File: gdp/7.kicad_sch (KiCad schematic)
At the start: 8 parts, among them IC1 74LS74, IC15A 74LS367, IC2 74LS42, IC21 74LS374, IC28 74LS374, IC35 74LS374, IC48 74LS374, IC9 74LS374

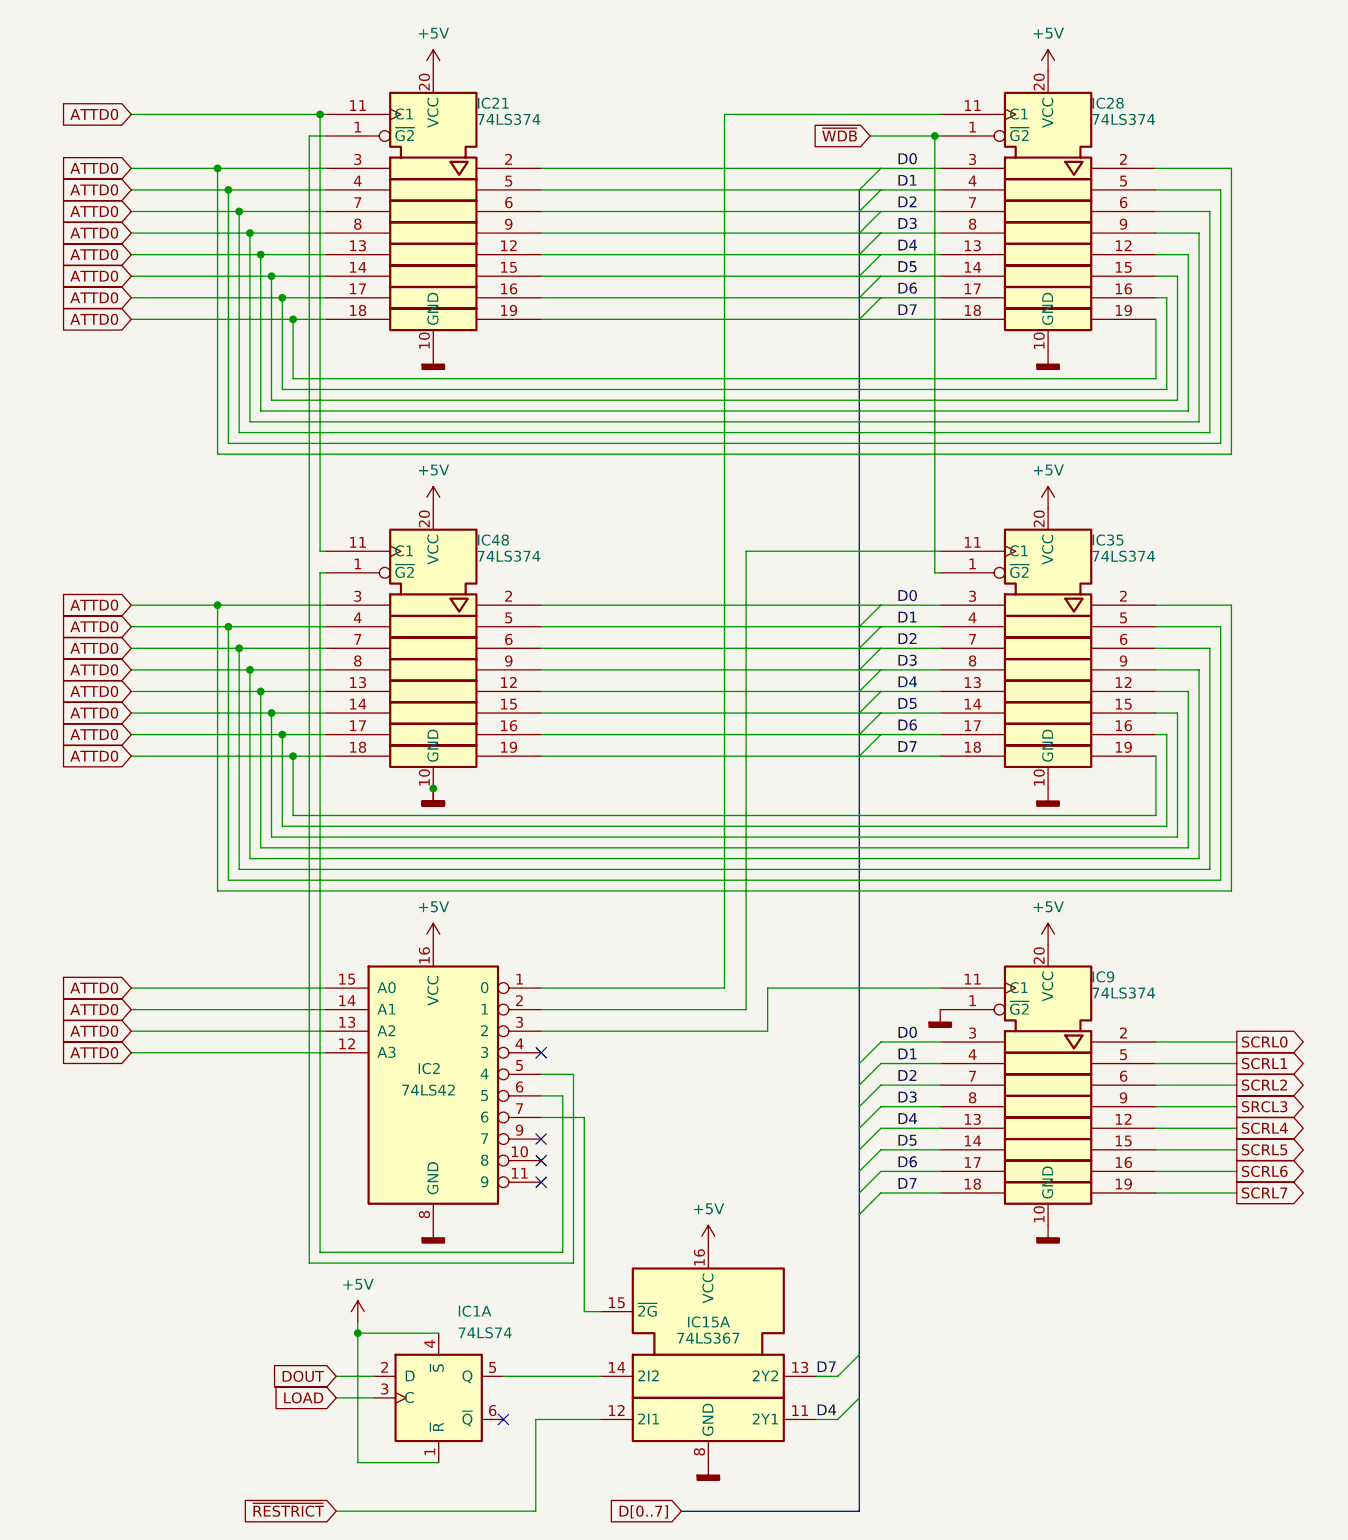
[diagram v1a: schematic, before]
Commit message: Fixes Sheet 7
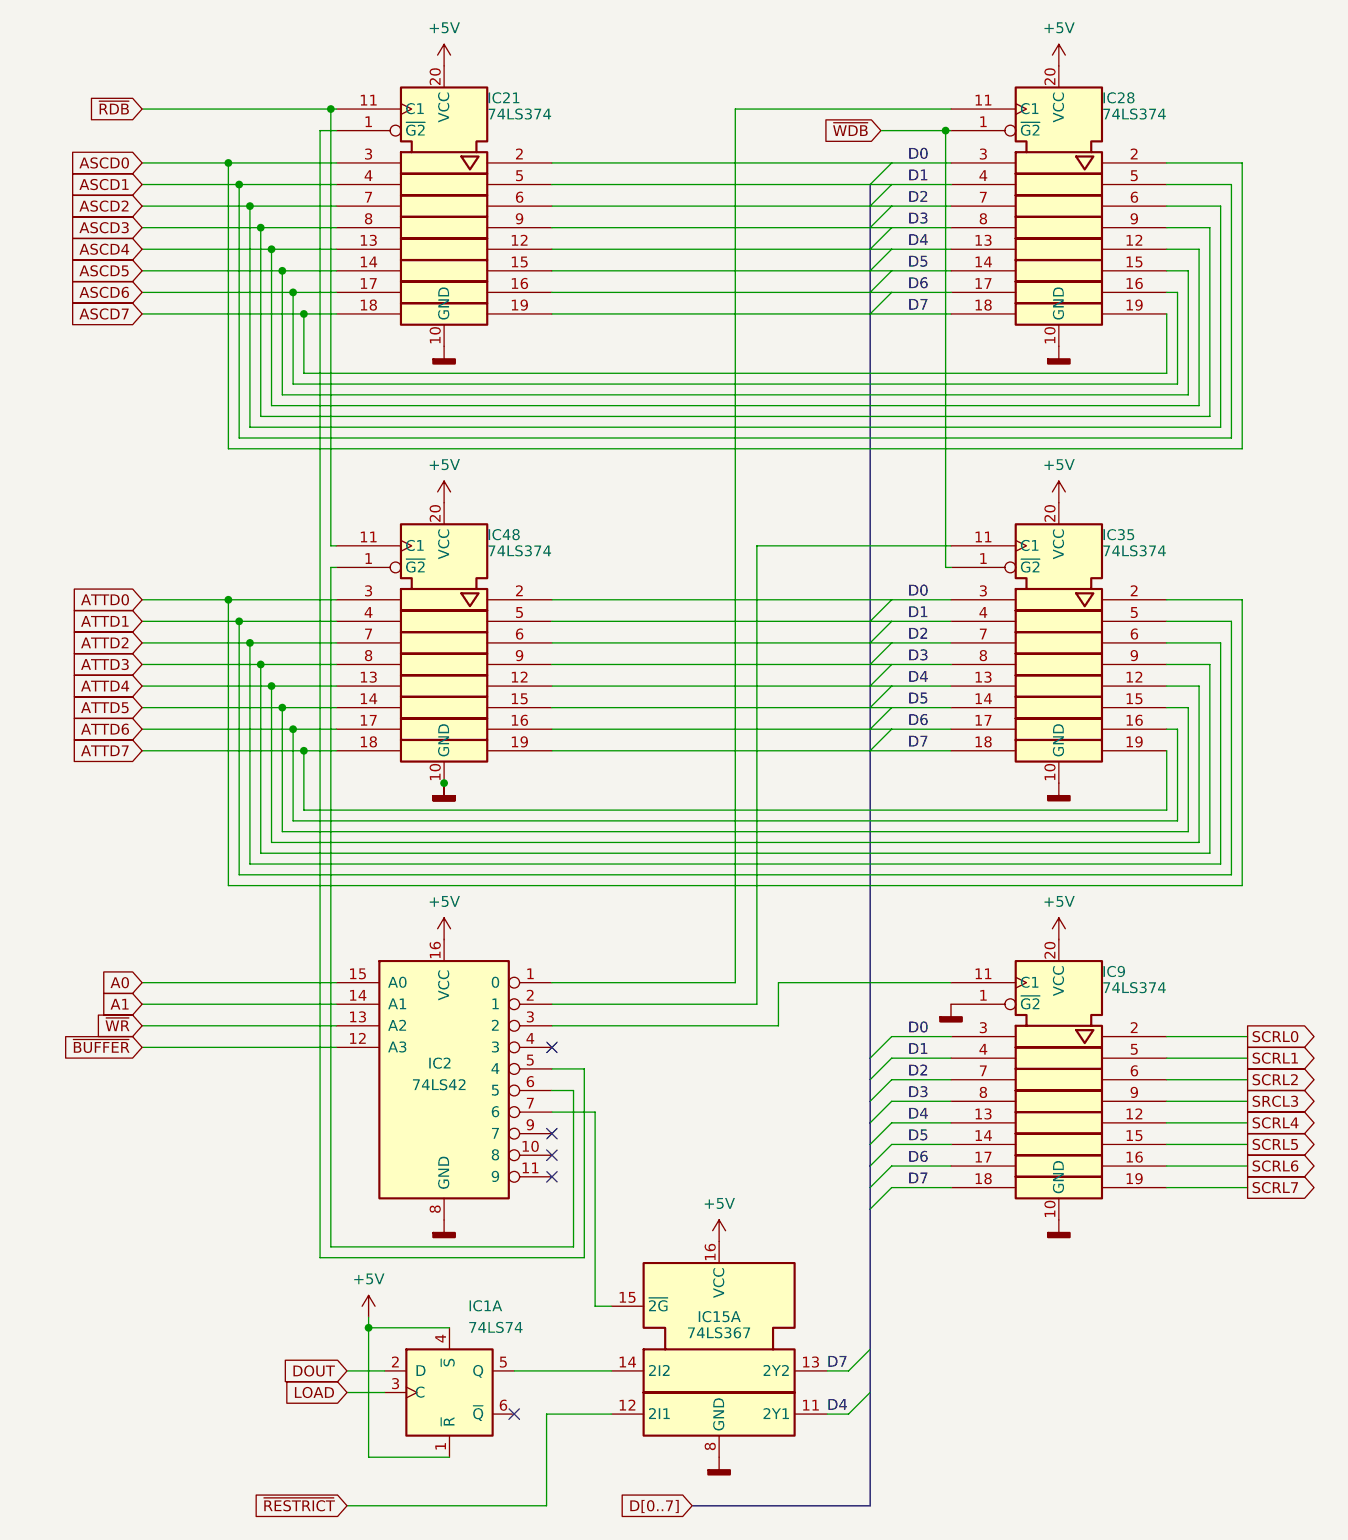
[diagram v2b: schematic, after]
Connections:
- net ATTD0: no longer IC2.12 (A3), IC2.13 (A2), IC2.14 (A1), IC2.15 (A0), IC21.11 (C1), IC21.13, IC21.14, IC21.17, IC21.18, IC21.3, IC21.4, IC21.7, IC21.8, IC28.12, IC28.15, IC28.16, IC28.19, IC28.2, IC28.5, IC28.6, IC28.9, IC35.12, IC35.15, IC35.16, IC35.19, IC35.5, IC35.6, IC35.9, IC48.11 (C1), IC48.13, IC48.14, IC48.17, IC48.18, IC48.4, IC48.7, IC48.8
- new net A0: IC2.15 (A0)
- new net A1: IC2.14 (A1)
- new net ASCD0: IC21.3, IC28.2
- new net ASCD1: IC21.4, IC28.5
- new net ASCD2: IC21.7, IC28.6
- new net ASCD3: IC21.8, IC28.9
- new net ASCD4: IC21.13, IC28.12
- new net ASCD5: IC21.14, IC28.15
- new net ASCD6: IC21.17, IC28.16
- new net ASCD7: IC21.18, IC28.19
- new net ATTD1: IC35.5, IC48.4
- new net ATTD2: IC35.6, IC48.7
- new net ATTD3: IC35.9, IC48.8
- new net ATTD4: IC35.12, IC48.13
- new net ATTD5: IC35.15, IC48.14
- new net ATTD6: IC35.16, IC48.17
- new net ATTD7: IC35.19, IC48.18
- new net ~{BUFFER}: IC2.12 (A3)
- new net ~{RDB}: IC21.11 (C1), IC48.11 (C1)
- new net ~{WR}: IC2.13 (A2)
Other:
- moved on the sheet: IC15A, IC1A, IC2, IC21, IC28, IC35, IC48, IC9

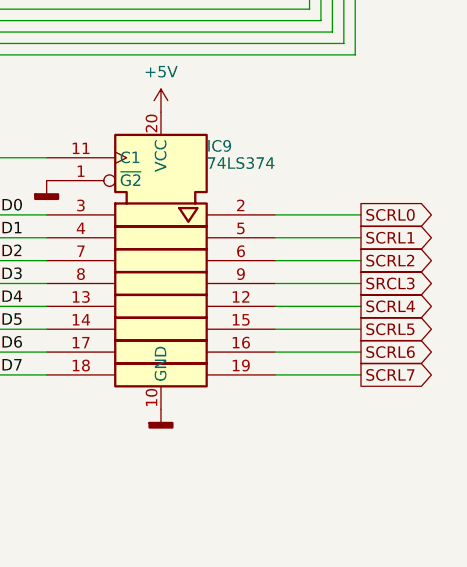
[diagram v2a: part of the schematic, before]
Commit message: Adds Sheet 14 (WIP)
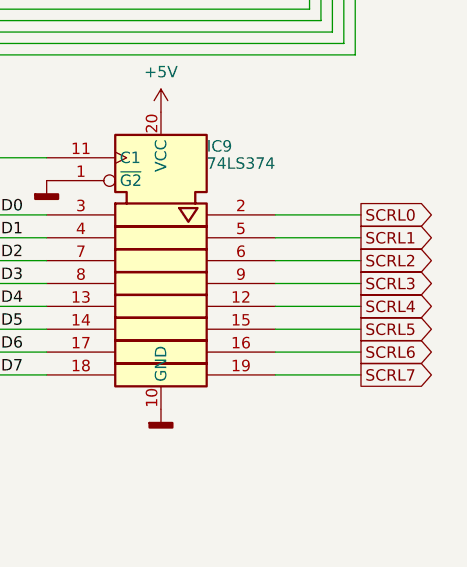
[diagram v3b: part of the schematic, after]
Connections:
- net SRCL3 renamed SCRL3
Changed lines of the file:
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@@
 		)
 	)
-	(global_label "SRCL3"
+	(global_label "SCRL3"
 		(shape output)
 		(at 213.995 140.335 0)

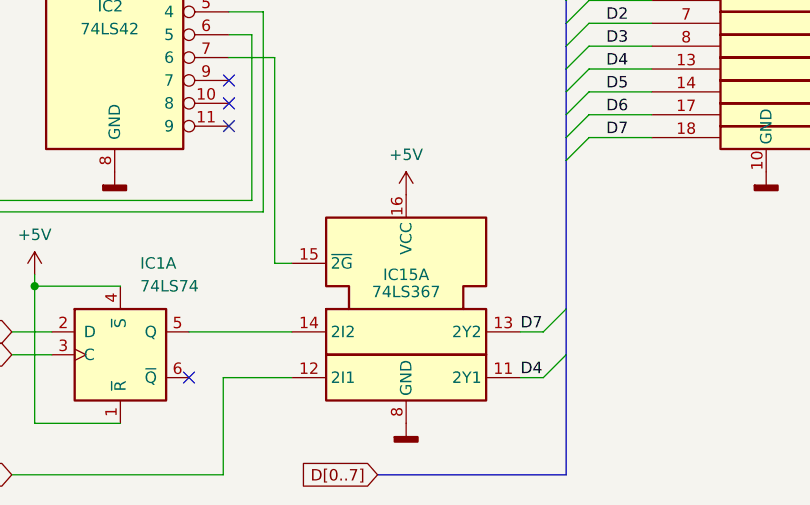
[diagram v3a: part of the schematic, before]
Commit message: Fixes IC15
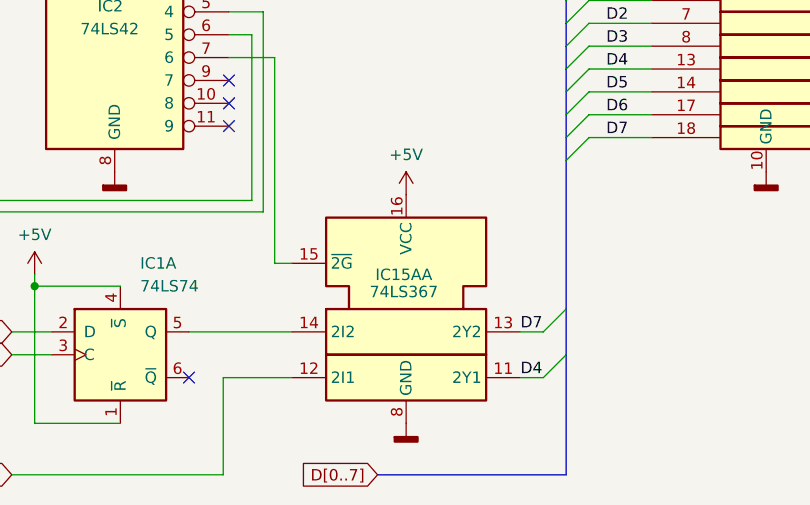
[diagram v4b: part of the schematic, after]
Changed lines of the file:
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@@
 		(dnp no)
 		(property "Reference" "IC15A"
-			(at 151.765 165.735 0)
+			(at 151.511 165.735 0)
 			(effects
 				(font
@@
 		)
 		(property "Value" "74LS367"
-			(at 151.765 167.64 0)
+			(at 151.511 167.64 0)
 			(effects
 				(font
@@
 		)
 		(property "Footprint" ""
-			(at 151.765 141.605 0)
+			(at 201.295 188.595 0)
 			(effects
 				(font
@@
 		)
 		(property "Datasheet" ""
-			(at 151.765 141.605 0)
+			(at 201.295 188.595 0)
 			(effects
 				(font
@@
 		)
 		(property "Description" ""
-			(at 151.765 169.545 0)
+			(at 151.511 167.005 0)
 			(effects
 				(font
@@
 		(pin "15"
 		)
+		(pin "10"
+		)
+		(pin "20"
+		)
+		(pin "1"
+		)
+		(pin "10"
+		)
+		(pin "2"
+		)
+		(pin "3"
+		)
+		(pin "16"
+		)
+		(pin "14"
+		)
+		(pin "4"
+		)
+		(pin "11"
+		)
+		(pin "8"
+		)
+		(pin "15"
+		)
+		(pin "7"
+		)
+		(pin "5"
+		)
+		(pin "13"
+		)
+		(pin "9"
+		)
+		(pin "12"
+		)
+		(pin "6"
+		)
 		(instances
 			(project "7"
@@
 			(project "gdp"
 				(path "/95aff260-2720-4733-a81d-a7a2136fdd14/953bb077-6bb4-4683-bd3b-895ed53ec170"
-					(reference "IC15A")
+					(reference "IC15")
 					(unit 1)
 				)
+				(path "/95aff260-2720-4733-a81d-a7a2136fdd14/d6b86f16-da3f-4420-ad10-a48d1b11a79a"
+					(reference "IC15")
+					(unit 1)
+				)

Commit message: Initial footprint assignment
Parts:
- IC1: footprint (none) -> Package_DIP:DIP-14_W7.62mm
- IC15A: footprint (none) -> Package_DIP:DIP-16_W7.62mm
- IC21, IC28, IC35, IC48, IC9: footprint (none) -> Package_DIP:DIP-20_W7.62mm
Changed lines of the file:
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@@
 			(project "gdp"
 				(path "/95aff260-2720-4733-a81d-a7a2136fdd14/953bb077-6bb4-4683-bd3b-895ed53ec170"
-					(reference "#PWR044")
+					(reference "#PWR088")
 					(unit 1)
 				)
@@
 			(project "gdp"
 				(path "/95aff260-2720-4733-a81d-a7a2136fdd14/953bb077-6bb4-4683-bd3b-895ed53ec170"
-					(reference "#PWR032")
+					(reference "#PWR0100")
 					(unit 1)
 				)
@@
 			(project "gdp"
 				(path "/95aff260-2720-4733-a81d-a7a2136fdd14/953bb077-6bb4-4683-bd3b-895ed53ec170"
-					(reference "#PWR034")
+					(reference "#PWR094")
 					(unit 1)
 				)
@@
 			(project "gdp"
 				(path "/95aff260-2720-4733-a81d-a7a2136fdd14/953bb077-6bb4-4683-bd3b-895ed53ec170"
-					(reference "#PWR028")
+					(reference "#PWR091")
 					(unit 1)
 				)
@@
 			)
 		)
-		(property "Footprint" ""
+		(property "Footprint" "Package_DIP:DIP-20_W7.62mm"
 			(at 191.77 136.525 0)
 			(effects
@@
 			)
 		)
-		(property "Datasheet" "https://www.digchip.com/datasheets/download_datasheet.php?id=369790&part-number=HEF40374BDB"
+		(property "Datasheet" "N/A"
 			(at 191.77 136.525 0)
 			(effects
@@
 			)
 		)
-		(property "Description" ""
+		(property "Description" "N/A"
 			(at 191.77 136.525 0)
 			(effects
@@
 			(project "gdp"
 				(path "/95aff260-2720-4733-a81d-a7a2136fdd14/953bb077-6bb4-4683-bd3b-895ed53ec170"
-					(reference "IC9")
+					(reference "IC45")
 					(unit 1)
 				)
@@
 			(project "gdp"
 				(path "/95aff260-2720-4733-a81d-a7a2136fdd14/953bb077-6bb4-4683-bd3b-895ed53ec170"
-					(reference "#PWR040")
+					(reference "#PWR0101")
 					(unit 1)
 				)
@@
 			(project "gdp"
 				(path "/95aff260-2720-4733-a81d-a7a2136fdd14/953bb077-6bb4-4683-bd3b-895ed53ec170"
-					(reference "#PWR029")
+					(reference "#PWR089")
 					(unit 1)
 				)
@@
 			(project "gdp"
 				(path "/95aff260-2720-4733-a81d-a7a2136fdd14/953bb077-6bb4-4683-bd3b-895ed53ec170"
-					(reference "#PWR033")
+					(reference "#PWR098")
 					(unit 1)
 				)
@@
 			)
 		)
-		(property "Footprint" ""
+		(property "Footprint" "Package_DIP:DIP-20_W7.62mm"
 			(at 119.38 33.655 0)
 			(effects
@@
 			)
 		)
-		(property "Datasheet" "https://www.digchip.com/datasheets/download_datasheet.php?id=369790&part-number=HEF40374BDB"
+		(property "Datasheet" "N/A"
 			(at 119.38 33.655 0)
 			(effects
@@
 			)
 		)
-		(property "Description" ""
+		(property "Description" "N/A"
 			(at 119.38 33.655 0)
 			(effects
@@
 			(project "gdp"
 				(path "/95aff260-2720-4733-a81d-a7a2136fdd14/953bb077-6bb4-4683-bd3b-895ed53ec170"
-					(reference "IC21")
+					(reference "IC38")
 					(unit 1)
 				)
@@
 			)
 		)
-		(property "Footprint" ""
+		(property "Footprint" "Package_DIP:DIP-14_W7.62mm"
 			(at 120.015 174.625 0)
 			(effects
@@
 			)
 		)
-		(property "Datasheet" "74xx/74hc_hct74.pdf"
+		(property "Datasheet" "N/A"
 			(at 120.015 174.625 0)
 			(effects
@@
 			)
 		)
-		(property "Description" ""
+		(property "Description" "N/A"
 			(at 120.015 174.625 0)
 			(effects
@@
 			(project "gdp"
 				(path "/95aff260-2720-4733-a81d-a7a2136fdd14/953bb077-6bb4-4683-bd3b-895ed53ec170"
-					(reference "IC1")
+					(reference "IC41")
 					(unit 1)
 				)
@@
 			(project "gdp"
 				(path "/95aff260-2720-4733-a81d-a7a2136fdd14/953bb077-6bb4-4683-bd3b-895ed53ec170"
-					(reference "#PWR031")
+					(reference "#PWR093")
 					(unit 1)
 				)
@@
 			)
 		)
-		(property "Datasheet" "http://www.ti.com/lit/gpn/sn74LS42"
+		(property "Datasheet" "N/A"
 			(at 119.38 136.525 0)
 			(effects
@@
 			)
 		)
-		(property "Description" ""
+		(property "Description" "N/A"
 			(at 119.38 136.525 0)
 			(effects
@@
 			(project "gdp"
 				(path "/95aff260-2720-4733-a81d-a7a2136fdd14/953bb077-6bb4-4683-bd3b-895ed53ec170"
-					(reference "IC2")
+					(reference "IC40")
 					(unit 1)
 				)
@@
 			(project "gdp"
 				(path "/95aff260-2720-4733-a81d-a7a2136fdd14/953bb077-6bb4-4683-bd3b-895ed53ec170"
-					(reference "#PWR039")
+					(reference "#PWR099")
 					(unit 1)
 				)
@@
 			(project "gdp"
 				(path "/95aff260-2720-4733-a81d-a7a2136fdd14/953bb077-6bb4-4683-bd3b-895ed53ec170"
-					(reference "#PWR038")
+					(reference "#PWR095")
 					(unit 1)
 				)
@@
 			(project "gdp"
 				(path "/95aff260-2720-4733-a81d-a7a2136fdd14/953bb077-6bb4-4683-bd3b-895ed53ec170"
-					(reference "#PWR046")
+					(reference "#PWR0102")
 					(unit 1)
 				)
@@
 			)
 		)
-		(property "Footprint" ""
+		(property "Footprint" "Package_DIP:DIP-20_W7.62mm"
 			(at 191.77 33.655 0)
 			(effects
@@
 			)
 		)
-		(property "Datasheet" "https://www.digchip.com/datasheets/download_datasheet.php?id=369790&part-number=HEF40374BDB"
+		(property "Datasheet" "N/A"
 			(at 191.77 33.655 0)
 			(effects
@@
 			)
 		)
-		(property "Description" ""
+		(property "Description" "N/A"
 			(at 191.77 33.655 0)
 			(effects
@@
 			(project "gdp"
 				(path "/95aff260-2720-4733-a81d-a7a2136fdd14/953bb077-6bb4-4683-bd3b-895ed53ec170"
-					(reference "IC28")
+					(reference "IC43")
 					(unit 1)
 				)
@@
 			(project "gdp"
 				(path "/95aff260-2720-4733-a81d-a7a2136fdd14/953bb077-6bb4-4683-bd3b-895ed53ec170"
-					(reference "#PWR045")
+					(reference "#PWR090")
 					(unit 1)
 				)
@@
 			(project "gdp"
 				(path "/95aff260-2720-4733-a81d-a7a2136fdd14/953bb077-6bb4-4683-bd3b-895ed53ec170"
-					(reference "#PWR037")
+					(reference "#PWR087")
 					(unit 1)
 				)
@@
 			)
 		)
-		(property "Footprint" ""
+		(property "Footprint" "Package_DIP:DIP-20_W7.62mm"
 			(at 119.38 85.09 0)
 			(effects
@@
 			)
 		)
-		(property "Datasheet" "https://www.digchip.com/datasheets/download_datasheet.php?id=369790&part-number=HEF40374BDB"
+		(property "Datasheet" "N/A"
 			(at 119.38 85.09 0)
 			(effects
@@
 			)
 		)
-		(property "Description" ""
+		(property "Description" "N/A"
 			(at 119.38 85.09 0)
 			(effects
@@
 			(project "gdp"
 				(path "/95aff260-2720-4733-a81d-a7a2136fdd14/953bb077-6bb4-4683-bd3b-895ed53ec170"
-					(reference "IC48")
+					(reference "IC39")
 					(unit 1)
 				)
@@
 			(project "gdp"
 				(path "/95aff260-2720-4733-a81d-a7a2136fdd14/953bb077-6bb4-4683-bd3b-895ed53ec170"
-					(reference "#PWR041")
+					(reference "#PWR0103")
 					(unit 1)
 				)
@@
 			)
 		)
-		(property "Footprint" ""
+		(property "Footprint" "Package_DIP:DIP-20_W7.62mm"
 			(at 191.77 85.09 0)
 			(effects
@@
 			)
 		)
-		(property "Datasheet" "https://www.digchip.com/datasheets/download_datasheet.php?id=369790&part-number=HEF40374BDB"
+		(property "Datasheet" "N/A"
 			(at 191.77 85.09 0)
 			(effects
@@
 			)
 		)
-		(property "Description" ""
+		(property "Description" "N/A"
 			(at 191.77 85.09 0)
 			(effects
@@
 			(project "gdp"
 				(path "/95aff260-2720-4733-a81d-a7a2136fdd14/953bb077-6bb4-4683-bd3b-895ed53ec170"
-					(reference "IC35")
+					(reference "IC44")
 					(unit 1)
 				)
@@
 			)
 		)
-		(property "Footprint" ""
+		(property "Footprint" "Package_DIP:DIP-16_W7.62mm"
 			(at 201.295 188.595 0)
 			(effects
@@
 			)
 		)
-		(property "Datasheet" ""
+		(property "Datasheet" "N/A"
 			(at 201.295 188.595 0)
 			(effects
@@
 			)
 		)
-		(property "Description" ""
+		(property "Description" "N/A"
 			(at 151.511 167.005 0)
 			(effects
@@
 			(project "gdp"
 				(path "/95aff260-2720-4733-a81d-a7a2136fdd14/953bb077-6bb4-4683-bd3b-895ed53ec170"
-					(reference "IC15")
+					(reference "IC42")
 					(unit 1)
 				)
@@
 			(project "gdp"
 				(path "/95aff260-2720-4733-a81d-a7a2136fdd14/953bb077-6bb4-4683-bd3b-895ed53ec170"
-					(reference "#PWR030")
+					(reference "#PWR092")
 					(unit 1)
 				)
@@
 			(project "gdp"
 				(path "/95aff260-2720-4733-a81d-a7a2136fdd14/953bb077-6bb4-4683-bd3b-895ed53ec170"
-					(reference "#PWR035")
+					(reference "#PWR097")
 					(unit 1)
 				)
@@
 			(project "gdp"
 				(path "/95aff260-2720-4733-a81d-a7a2136fdd14/953bb077-6bb4-4683-bd3b-895ed53ec170"
-					(reference "#PWR036")
-					(unit 1)
-				)
+					(reference "#PWR096")
+					(unit 1)
+				)
